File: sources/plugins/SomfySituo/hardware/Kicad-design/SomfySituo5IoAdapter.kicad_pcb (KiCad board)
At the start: 2 copper layers, 25.4 x 21.8 mm, 30 parts, among them J1 USB_OTG, J10 Conn_01x01, J11 Conn_01x01, J12 Conn_01x01, J13 Conn_01x01, J15 ICSP, J2 Conn_01x01, J3 Conn_01x01, J4 Conn_01x01, J5 Conn_01x01, J6 Conn_01x01, J7 Conn_01x01, J8 Conn_01x01, J9 Conn_01x01, U1 FT230X, U2 PIC16F688

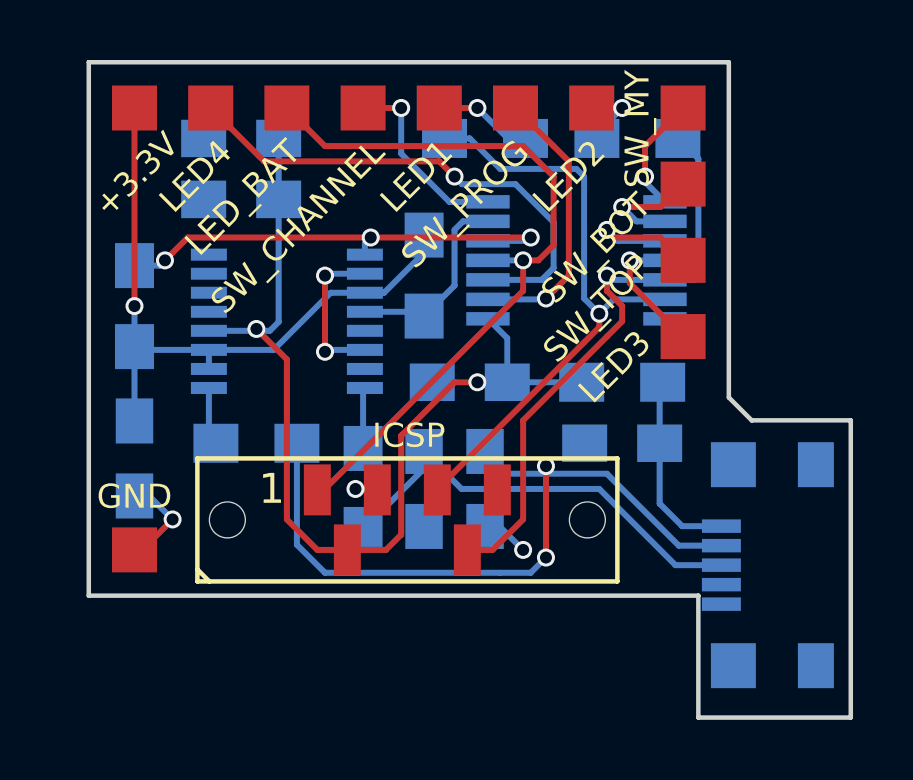
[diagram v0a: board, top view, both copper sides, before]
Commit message: Send PCB to factoring
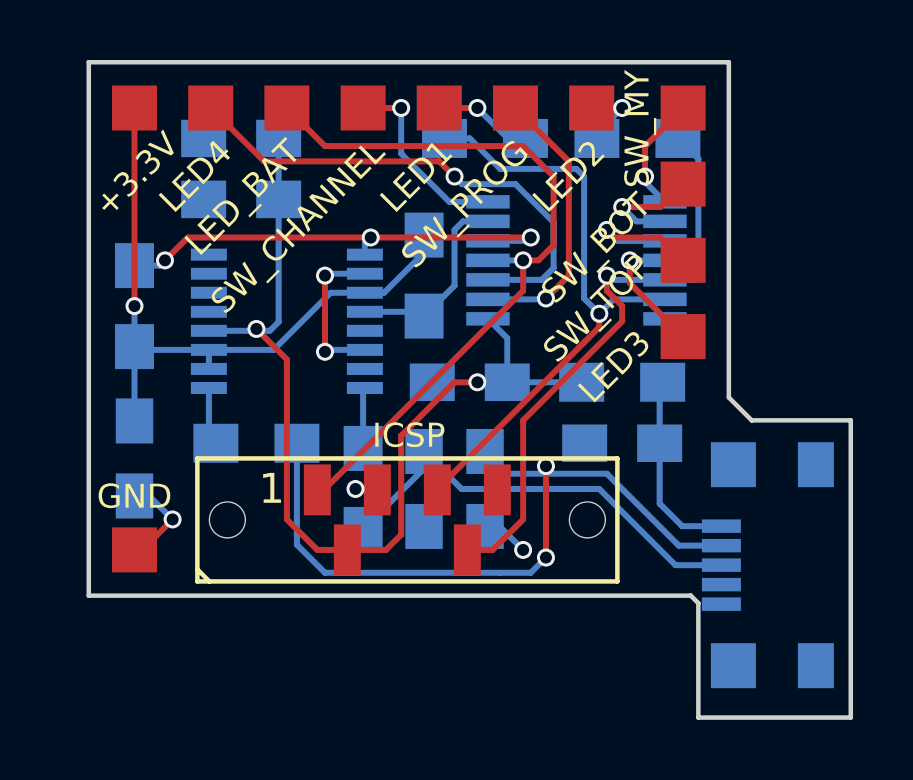
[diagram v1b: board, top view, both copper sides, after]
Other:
- outline, holes or cut-outs redrawn
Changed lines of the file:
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@@
     (links 57)
     (no_connects 0)
-    (area 108.128999 110.160999 133.679001 132.155001)
+    (area 90.194001 97.376 153.138 141.384001)
     (thickness 1.6)
-    (drawings 39)
+    (drawings 41)
     (tracks 194)
     (zones 0)
@@
     (visible_elements 7FFFFF7F)
     (pcbplotparams
-      (layerselection 0x00030_80000001)
+      (layerselection 0x010f0_80000001)
       (usegerberextensions false)
       (excludeedgelayer true)
@@
       (outputformat 1)
       (mirror false)
-      (drillshape 1)
+      (drillshape 0)
       (scaleselection 1)
-      (outputdirectory ""))
+      (outputdirectory out/))
   )
   (net 0 "")
@@
       (net 2 GND))
   )
+  (gr_line (start 128.27 128.016) (end 108.204 128.016) (angle 90) (layer Edge.Cuts) (width 0.15))
+  (gr_line (start 128.524 128.27) (end 128.27 128.016) (angle 90) (layer Edge.Cuts) (width 0.15))
+  (gr_line (start 128.524 132.08) (end 128.524 128.27) (angle 90) (layer Edge.Cuts) (width 0.15))
+  (dimension 25.4 (width 0.3) (layer Cmts.User)
+    (gr_text "25,400 mm" (at 120.904 98.726) (layer Cmts.User)
+      (effects (font (size 1.5 1.5) (thickness 0.3)))
+    )
+    (feature1 (pts (xy 133.604 103.886) (xy 133.604 97.376)))
+    (feature2 (pts (xy 108.204 103.886) (xy 108.204 97.376)))
+    (crossbar (pts (xy 108.204 100.076) (xy 133.604 100.076)))
+    (arrow1a (pts (xy 133.604 100.076) (xy 132.477496 100.662421)))
+    (arrow1b (pts (xy 133.604 100.076) (xy 132.477496 99.489579)))
+    (arrow2a (pts (xy 108.204 100.076) (xy 109.330504 100.662421)))
+    (arrow2b (pts (xy 108.204 100.076) (xy 109.330504 99.489579)))
+  )
   (gr_circle (center 128.27 124.841) (end 128.397 124.841) (layer B.SilkS) (width 0.2))
   (gr_circle (center 117.729 115.697) (end 117.856 115.697) (layer B.SilkS) (width 0.2))
@@
   )
   (gr_line (start 108.204 110.236) (end 129.54 110.236) (angle 90) (layer Edge.Cuts) (width 0.15))
-  (gr_line (start 108.204 128.016) (end 128.524 128.016) (angle 90) (layer Edge.Cuts) (width 0.15))
   (gr_line (start 108.204 110.236) (end 108.204 128.016) (angle 90) (layer Edge.Cuts) (width 0.15))
   (dimension 21.844 (width 0.3) (layer Cmts.User)
@@
     (effects (font (size 1 1) (thickness 0.2)))
   )
-  (gr_line (start 128.524 132.08) (end 128.524 128.016) (angle 90) (layer Edge.Cuts) (width 0.15))
   (gr_line (start 133.604 132.08) (end 128.524 132.08) (angle 90) (layer Edge.Cuts) (width 0.15))
   (segment (start 116.824 126.492) (end 115.824 126.492) (width 0.2) (layer F.Cu) (net 1))
@@
       (pts
         (xy 108.204 110.236) (xy 129.54 110.236) (xy 129.54 121.412) (xy 130.302 122.174) (xy 133.604 122.174)
-        (xy 133.604 132.08) (xy 128.524 132.08) (xy 128.524 128.016) (xy 108.204 128.016)
+        (xy 133.604 132.08) (xy 128.524 132.08) (xy 128.524 128.27) (xy 128.27 128.016) (xy 108.204 128.016)
       )
     )
@@
       (pts
         (xy 108.204 110.236) (xy 129.54 110.236) (xy 129.54 121.412) (xy 130.302 122.174) (xy 133.604 122.174)
-        (xy 133.604 132.08) (xy 128.524 132.08) (xy 128.524 128.016) (xy 108.204 128.016)
+        (xy 133.604 132.08) (xy 128.524 132.08) (xy 128.524 128.27) (xy 128.27 128.016) (xy 108.204 128.016)
       )
     )
